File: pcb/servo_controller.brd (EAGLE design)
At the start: 68.6 x 53.3 mm, 50 parts, among them IC2 PIC18F452, IC4 LM2937, U1 ARDUINOR3-DIMENSION

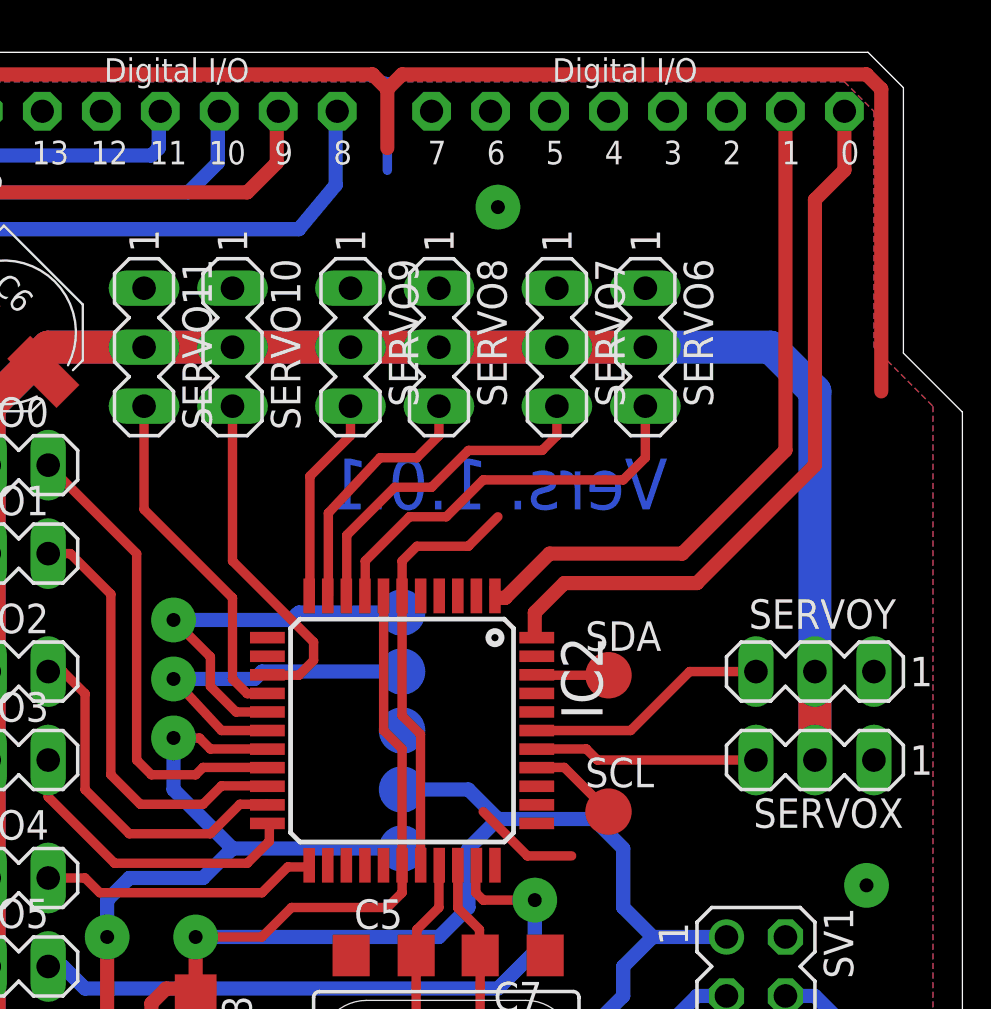
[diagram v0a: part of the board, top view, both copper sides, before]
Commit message: Update
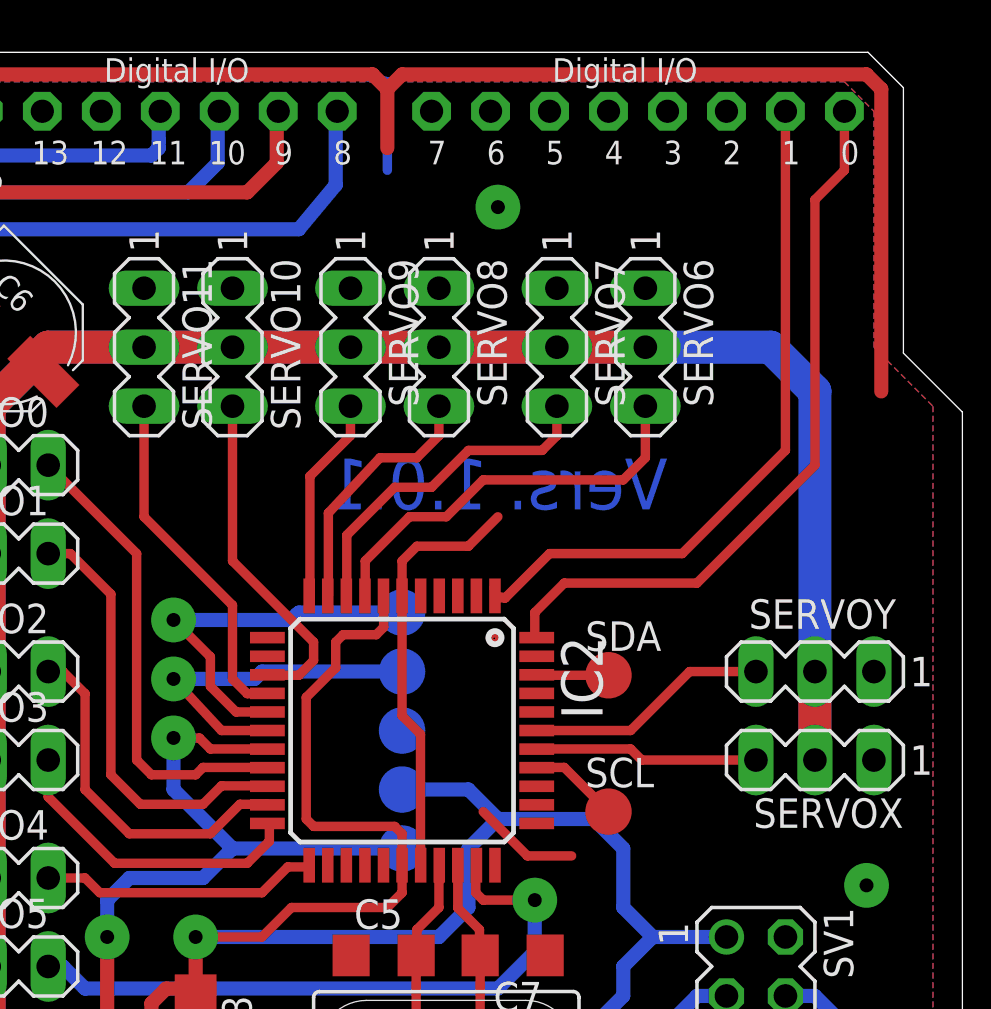
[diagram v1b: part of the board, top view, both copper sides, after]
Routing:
- net +5V: track 153.6 -> 159.2 mm
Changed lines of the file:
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@@
 <plain>
 <text x="55.88" y="33.655" size="2.1844" layer="16" font="vector" rot="MR0">Vers. 1.0.1</text>
+<circle x="48.41875" y="28.09875" radius="0.15875" width="0.4064" layer="1"/>
 </plain>
 <attributes>
@@
 <contactref element="IC2" pad="44"/>
 <contactref element="U1" pad="D0"/>
-<wire x1="63.5" y1="50.8" x2="63.5" y2="48.26" width="0.6096" layer="1"/>
-<wire x1="63.5" y1="48.26" x2="62.23" y2="46.99" width="0.6096" layer="1"/>
-<wire x1="62.23" y1="46.99" x2="62.23" y2="35.56" width="0.6096" layer="1"/>
-<wire x1="62.23" y1="35.56" x2="57.15" y2="30.48" width="0.6096" layer="1"/>
-<wire x1="57.15" y1="30.48" x2="51.435" y2="30.48" width="0.6096" layer="1"/>
-<wire x1="51.435" y1="30.48" x2="50.165" y2="29.21" width="0.6096" layer="1"/>
-<wire x1="50.165" y1="29.21" x2="50.165" y2="28.2575" width="0.6096" layer="1"/>
 <wire x1="50.165" y1="28.2575" x2="50.25" y2="28.13" width="0.4064" layer="1"/>
+<wire x1="63.5" y1="50.8" x2="63.5" y2="48.26" width="0.4064" layer="1"/>
+<wire x1="63.5" y1="48.26" x2="62.23" y2="46.99" width="0.4064" layer="1"/>
+<wire x1="62.23" y1="46.99" x2="62.23" y2="35.56" width="0.4064" layer="1"/>
+<wire x1="62.23" y1="35.56" x2="57.15" y2="30.48" width="0.4064" layer="1"/>
+<wire x1="57.15" y1="30.48" x2="51.435" y2="30.48" width="0.4064" layer="1"/>
+<wire x1="51.435" y1="30.48" x2="50.165" y2="29.21" width="0.4064" layer="1"/>
+<wire x1="50.165" y1="29.21" x2="50.165" y2="28.215" width="0.4064" layer="1"/>
+<wire x1="50.165" y1="28.215" x2="50.25" y2="28.13" width="0.4064" layer="1"/>
 </signal>
 <signal name="TX_FROM_ARDUINO">
@@
 <wire x1="48.45" y1="29.93" x2="48.41875" y2="30.32125" width="0.4064" layer="1"/>
 <contactref element="U1" pad="D1"/>
-<wire x1="60.96" y1="50.8" x2="60.96" y2="36.195" width="0.6096" layer="1"/>
-<wire x1="60.96" y1="36.195" x2="56.515" y2="31.75" width="0.6096" layer="1"/>
-<wire x1="56.515" y1="31.75" x2="50.8" y2="31.75" width="0.6096" layer="1"/>
-<wire x1="50.8" y1="31.75" x2="48.895" y2="29.845" width="0.6096" layer="1"/>
 <wire x1="48.895" y1="29.845" x2="48.45" y2="29.93" width="0.4064" layer="1"/>
-<wire x1="48.895" y1="29.845" x2="48.5775" y2="29.845" width="0.6096" layer="1"/>
+<wire x1="60.96" y1="50.8" x2="60.96" y2="36.195" width="0.4064" layer="1"/>
+<wire x1="60.96" y1="36.195" x2="56.515" y2="31.75" width="0.4064" layer="1"/>
+<wire x1="56.515" y1="31.75" x2="50.8" y2="31.75" width="0.4064" layer="1"/>
+<wire x1="50.8" y1="31.75" x2="48.895" y2="29.845" width="0.4064" layer="1"/>
+<wire x1="48.895" y1="29.845" x2="48.535" y2="29.845" width="0.4064" layer="1"/>
+<wire x1="48.535" y1="29.845" x2="48.45" y2="29.93" width="0.4064" layer="1"/>
 </signal>
 <signal name="N$9">
@@
 <wire x1="37.7825" y1="25.7175" x2="38.6375" y2="25.7175" width="0.4064" layer="1"/>
 <wire x1="38.6375" y1="25.7175" x2="38.65" y2="25.73" width="0.4064" layer="1"/>
-<wire x1="33.3375" y1="38.1" x2="33.3375" y2="33.655" width="0.4064" layer="1"/>
-<wire x1="33.3375" y1="33.655" x2="37.1475" y2="29.845" width="0.4064" layer="1"/>
-<wire x1="37.1475" y1="29.845" x2="37.1475" y2="26.3525" width="0.4064" layer="1"/>
+<wire x1="33.3375" y1="38.1" x2="33.3375" y2="33.3375" width="0.4064" layer="1"/>
+<wire x1="33.3375" y1="33.3375" x2="37.1475" y2="29.5275" width="0.4064" layer="1"/>
+<wire x1="37.1475" y1="29.5275" x2="37.1475" y2="26.3525" width="0.4064" layer="1"/>
 <wire x1="37.1475" y1="26.3525" x2="37.7825" y2="25.7175" width="0.4064" layer="1"/>
 </signal>
@@
 <contactref element="IC2" pad="38"/>
 <wire x1="50.25" y1="23.33" x2="50.64125" y2="23.33625" width="0.4064" layer="1"/>
-<wire x1="50.64125" y1="23.33625" x2="52.3875" y2="23.33625" width="0.4064" layer="1"/>
-<wire x1="52.3875" y1="23.33625" x2="52.86375" y2="22.86" width="0.4064" layer="1"/>
-<wire x1="52.86375" y1="22.86" x2="59.69" y2="22.86" width="0.4064" layer="1"/>
+<wire x1="50.64125" y1="23.33625" x2="54.2925" y2="23.33625" width="0.4064" layer="1"/>
+<wire x1="54.2925" y1="23.33625" x2="54.76875" y2="22.86" width="0.4064" layer="1"/>
+<wire x1="54.76875" y1="22.86" x2="59.69" y2="22.86" width="0.4064" layer="1"/>
 </signal>
 <signal name="N$24">
@@
 <contactref element="IC3" pad="1"/>
 <contactref element="VDD" pad="TP"/>
-<wire x1="44.45" y1="18.33" x2="44.45" y2="23.33625" width="0.4064" layer="1"/>
-<wire x1="44.45" y1="23.33625" x2="43.65625" y2="24.13" width="0.4064" layer="1"/>
-<wire x1="43.65625" y1="24.13" x2="43.65625" y2="29.92375" width="0.4064" layer="1"/>
-<wire x1="43.65625" y1="29.92375" x2="43.65" y2="29.93" width="0.4064" layer="1"/>
+<wire x1="44.45" y1="18.33" x2="44.45" y2="19.685" width="0.4064" layer="1"/>
 <wire x1="44.45" y1="18.33" x2="44.45" y2="17.145" width="0.4064" layer="1"/>
 <wire x1="44.45" y1="17.145" x2="43.815" y2="16.51" width="0.4064" layer="1"/>
@@
 <wire x1="14.9225" y1="15.5575" x2="13.3375" y2="15.5575" width="0.6096" layer="1"/>
 <wire x1="13.3375" y1="15.5575" x2="13.6525" y2="15.56" width="0.6096" layer="1"/>
+<wire x1="44.45" y1="19.685" x2="44.1325" y2="20.0025" width="0.4064" layer="1"/>
+<wire x1="44.1325" y1="20.0025" x2="40.64" y2="20.0025" width="0.4064" layer="1"/>
+<wire x1="40.64" y1="20.0025" x2="40.3225" y2="20.32" width="0.4064" layer="1"/>
+<wire x1="40.3225" y1="20.32" x2="40.3225" y2="25.55875" width="0.4064" layer="1"/>
+<wire x1="40.3225" y1="25.55875" x2="41.5925" y2="26.82875" width="0.4064" layer="1"/>
+<wire x1="41.5925" y1="26.82875" x2="41.5925" y2="27.94" width="0.4064" layer="1"/>
+<wire x1="41.5925" y1="27.94" x2="41.91" y2="28.2575" width="0.4064" layer="1"/>
+<wire x1="41.91" y1="28.2575" x2="43.33875" y2="28.2575" width="0.4064" layer="1"/>
+<wire x1="43.33875" y1="28.2575" x2="43.65625" y2="28.575" width="0.4064" layer="1"/>
+<wire x1="43.65625" y1="28.575" x2="43.65625" y2="29.92375" width="0.4064" layer="1"/>
+<wire x1="43.65625" y1="29.92375" x2="43.65" y2="29.93" width="0.4064" layer="1"/>
 </signal>
 <signal name="GND">
